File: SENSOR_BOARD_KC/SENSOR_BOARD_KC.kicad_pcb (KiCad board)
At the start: 2 copper layers, 209 x 150 mm, 34 parts, among them SW2 SW_Push, SW3 SW_Push, SW4 SW_Push, SW5 SW_Push, U1 BP

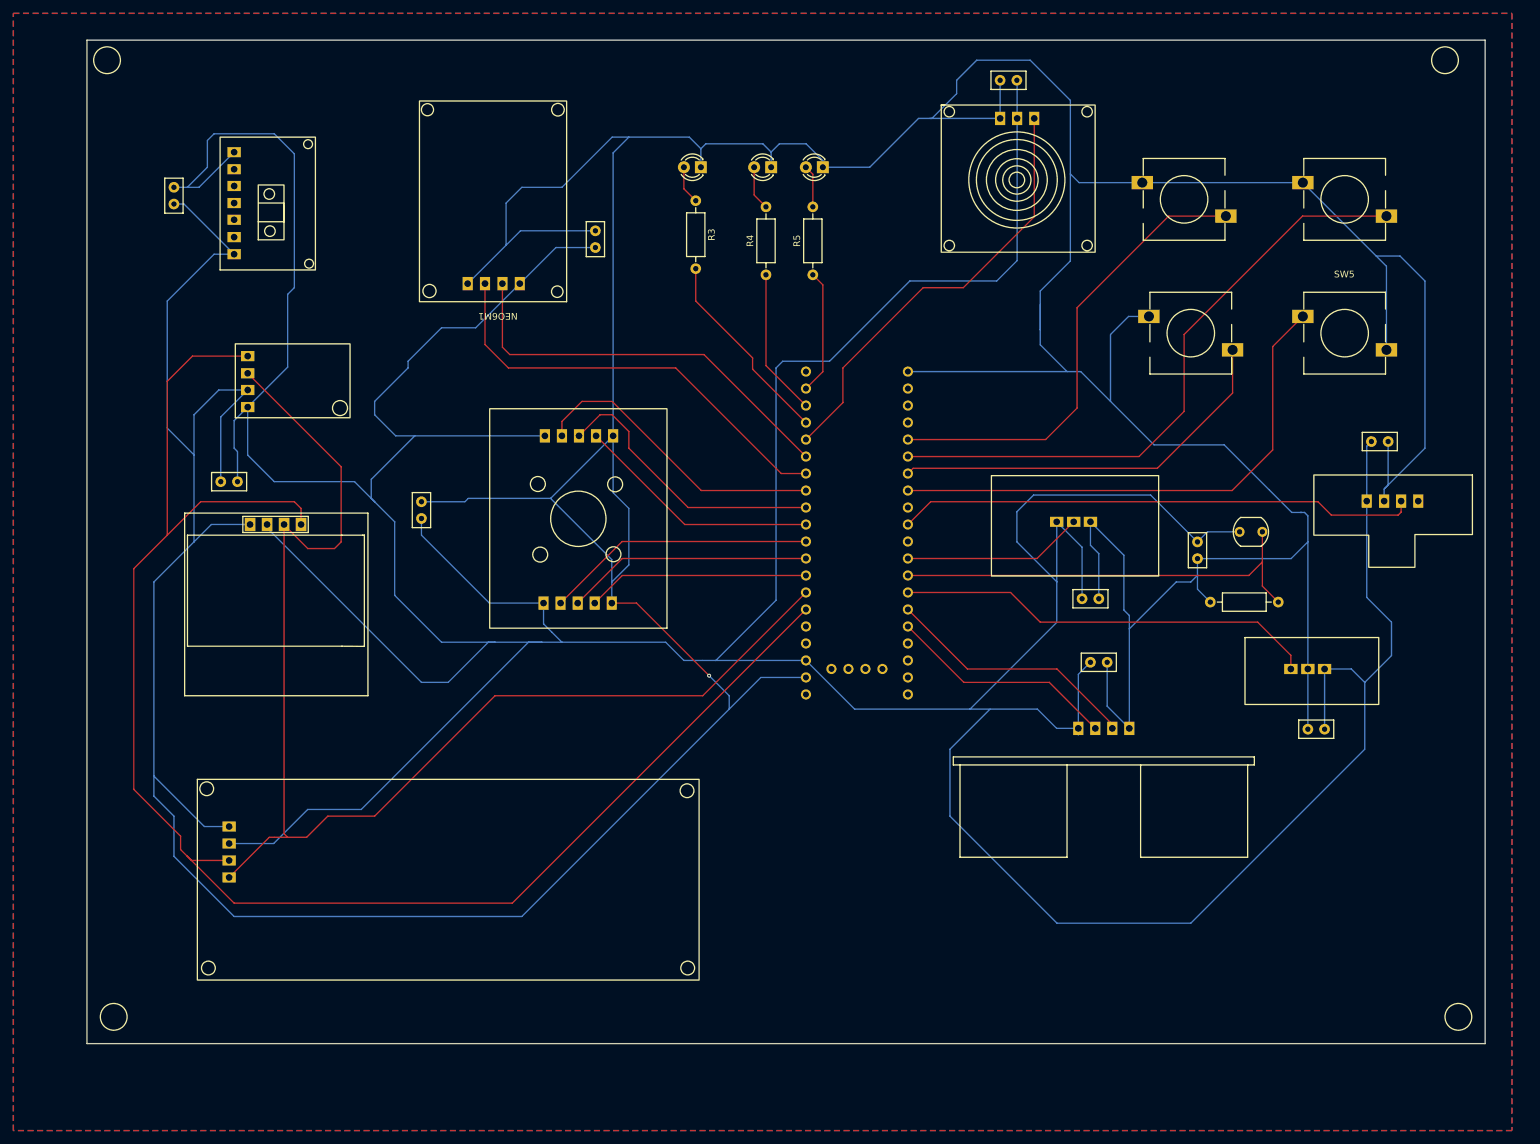
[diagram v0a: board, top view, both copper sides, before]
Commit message: Updates
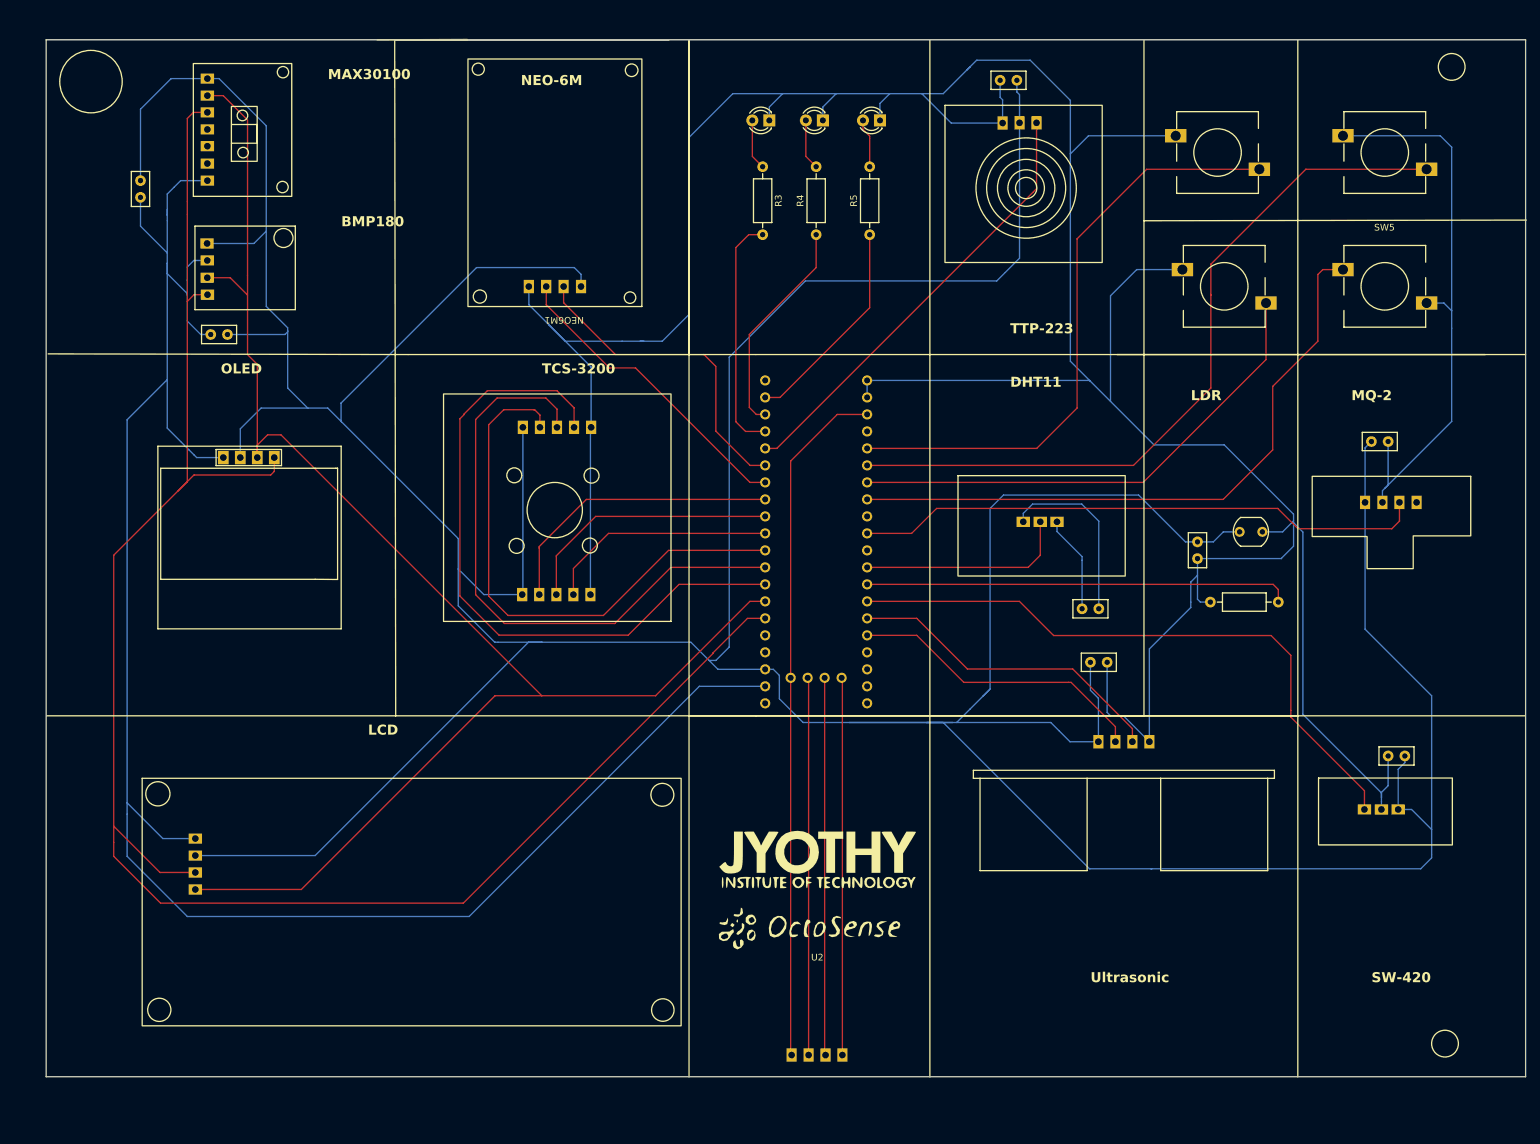
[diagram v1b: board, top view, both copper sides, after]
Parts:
- removed C6, C8: 0.1u, Capacitor_THT:C_Disc_D5.0mm_W2.5mm_P2.50mm
- added G***: LOGO, LOGO, F.Cu at (170.9, 152.2)
- added G***: LOGO, LOGO, F.Cu at (170.0, 159.3)
- added U2: ~, Sensor_footprints:STLINK_Connect, F.Cu at (171.2, 181.6)
- moved SW1 23.7 mm to (255.5, 145.0)
- moved C12 22.1 mm to (83.0, 74.0)
- moved BMP1 17.8 mm to (87.7, 64.0)
- moved C1 12.6 mm to (259.0, 137.0)
- moved D1 12.4 mm to (164.0, 42.0)
- moved MAX1 11.7 mm to (85.0, 44.0)
- moved R3 11.2 mm to (163.0, 48.9)
- moved D3 11.0 mm to (180.5, 42.0)
- moved OLED1 10.8 mm to (86.0, 103.0)
- moved D2 10.4 mm to (172.0, 42.0)
- moved R5 10.4 mm to (179.0, 59.1)
- moved NEO6M1 9.92 mm to (133.9, 52.6)
- moved R4 9.60 mm to (171.0, 59.1)
- moved SW3 9.22 mm to (256.0, 47.0)
- moved SW5 9.22 mm to (256.0, 67.0)
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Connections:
- U1 pad 3V3: unconnected-(U1-3.3V-Pad3V3) -> Net-(U1-3.3V)
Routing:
- net (no net): track 0.00 -> 112.9 mm
- net Net-(U1-3.3V): track 0.00 -> 103.2 mm
- net Net-(TCS1-OUT): track 33.3 -> 100.5 mm
- net Net-(TCS1-S2): track 36.9 -> 91.6 mm
- net Net-(TCS1-S3): track 40.5 -> 82.9 mm
- net Net-(BMP1-SCL): track 192.3 -> 229.9 mm
- net Net-(BMP1-SDA): track 234.9 -> 272.4 mm
- net Net-(BMP1-vcc): track 853.6 -> 820.7 mm
- net Net-(SW1-d0): track 63.2 -> 94.3 mm
- net Net-(SW2-Pad2): track 70.2 -> 90.7 mm
- net Net-(SW3-Pad2): track 93.2 -> 112.9 mm
- net Net-(NEO6M1-TX): track 65.1 -> 46.5 mm
- net Net-(SW5-Pad1): track 78.9 -> 96.8 mm
- net Net-(SW4-Pad2): track 60.0 -> 75.7 mm
- net Net-(R5-Pad1): track 18.7 -> 32.1 mm
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- removed copper zone on B.Cu, net (none)
- removed copper zone on F.Cu, net (none)
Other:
- board size 209 x 150 mm -> 221.2 x 155 mm
- board text added: "BMP180"
- board text added: "DHT11"
- board text added: "LCD"
- board text added: "LDR"
- board text added: "MAX30100"
- board text added: "MQ-2"
- board text added: "NEO-6M"
- board text added: "OLED"
- board text added: "SW-420"
- board text added: "TCS-3200"
- board text added: "TTP-223"
- board text added: "Ultrasonic"
